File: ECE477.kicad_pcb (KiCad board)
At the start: 2 copper layers, 88.9 x 88.9 mm, 55 parts, among them IC1 LP3852EMP-3.3_NOPB, IC2 BQ29330DBT, J1 P7805-2000-S, J10 Conn_01x01_Male, J11 Conn_01x01_Male, J2 Conn_01x05_Male, J3 Conn_01x05_Male, J4 Conn_01x05_Male, J5 Conn_01x05_Male, J6 Conn_01x05_Male, J7 Conn_01x05_Male, J8 Conn_01x05_Male, J9 Conn_01x01_Male, SW1 SW_Push_Dual, U1 STM32H7_LQFP144_T2

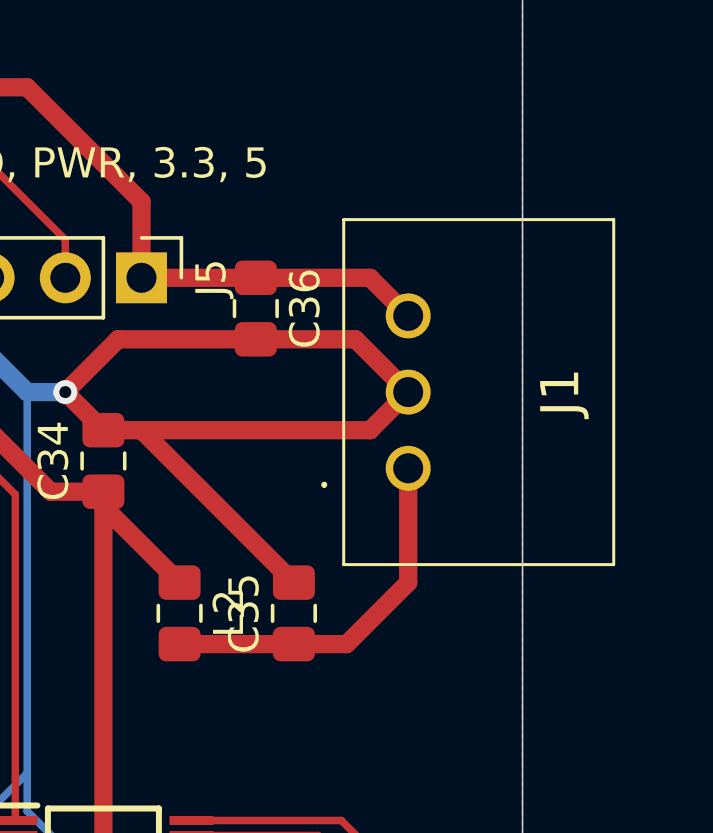
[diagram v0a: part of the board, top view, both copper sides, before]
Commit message: DRC corrections
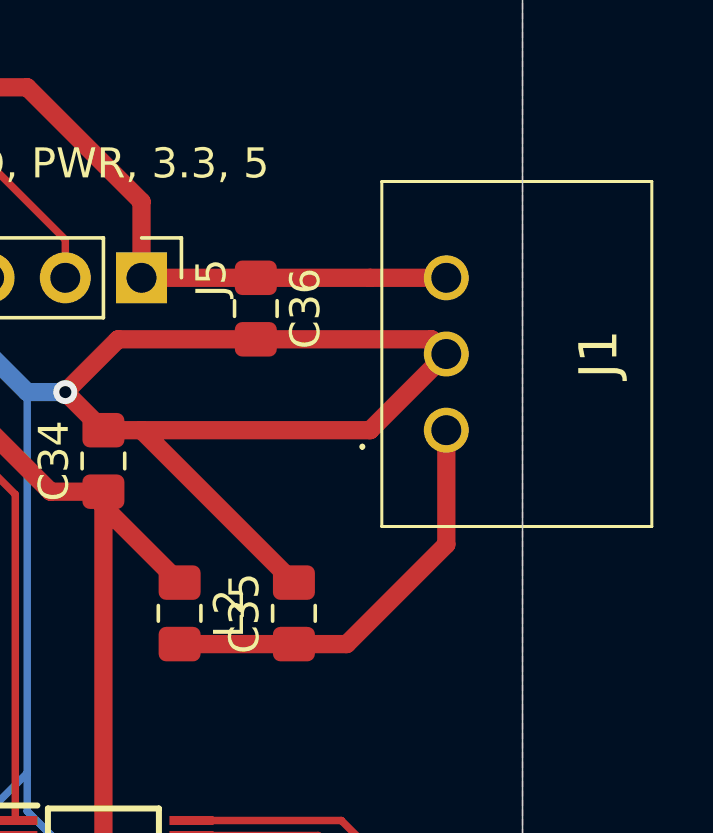
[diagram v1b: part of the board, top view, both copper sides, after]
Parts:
- moved J1 1.80 mm to (238.8, 69.8)
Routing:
- net GND: track 689.0 -> 691.6 mm
- net Net-(C35-Pad1): track 12.3 -> 14.1 mm
- net 5V: track 63.4 -> 64.1 mm
